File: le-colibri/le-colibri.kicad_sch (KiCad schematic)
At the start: 61 parts, among them SW1 CPG151101S11, SW10 CPG151101S11, SW11 CPG151101S11, SW12 CPG151101S11, SW13 CPG151101S11, SW14 CPG151101S11, SW15 CPG151101S11, SW16 CPG151101S11, SW17 CPG151101S11, SW18 CPG151101S11, SW19 CPG151101S11, SW2 CPG151101S11, SW20 CPG151101S11, SW21 CPG151101S11, SW22 CPG151101S11, SW23 CPG151101S11, SW24 CPG151101S11, SW25 CPG151101S11, SW26 CPG151101S11, SW27 CPG151101S11, SW28 CPG151101S11, SW29 CPG151101S11, SW3 CPG151101S11, SW30 CPG151101S11, SW4 CPG151101S11, SW5 CPG151101S11, SW6 CPG151101S11, SW7 CPG151101S11, SW8 CPG151101S11, SW9 CPG151101S11, U1 Seeeduino Xiao rp2040

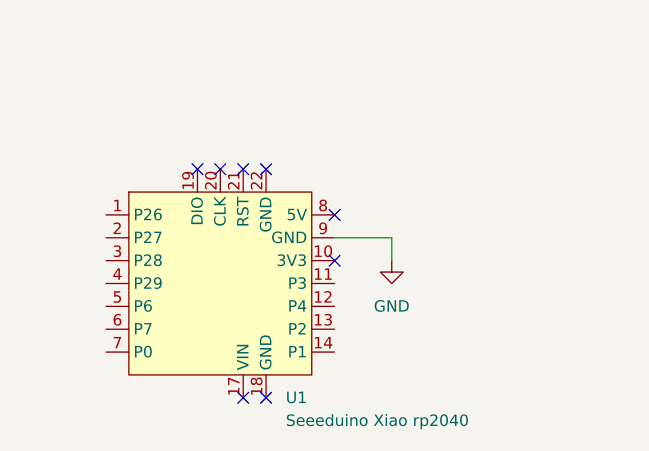
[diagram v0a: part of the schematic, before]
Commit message: "first" "release"
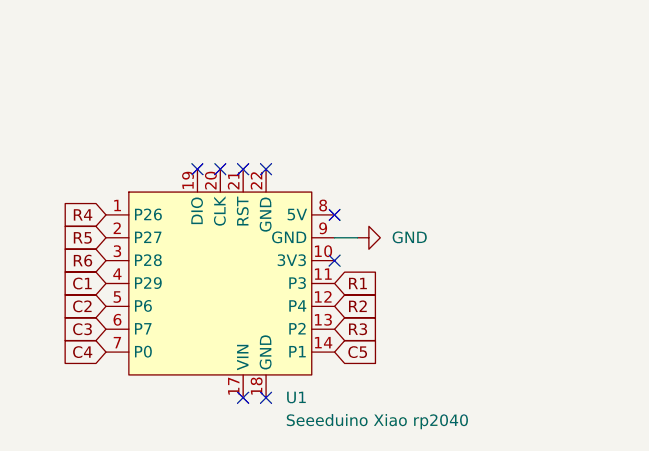
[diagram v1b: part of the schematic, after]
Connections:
- net C1: now also U1.4 (P29)
- net C2: now also U1.5 (P6)
- net C3: now also U1.6 (P7)
- net C4: now also U1.7 (P0)
- net C5: now also U1.14 (P1)
- net R1: now also U1.11 (P3)
- net R2: now also U1.12 (P4)
- net R3: now also U1.13 (P2)
- net R4: now also U1.1 (P26)
- net R5: now also U1.2 (P27)
- net R6: now also U1.3 (P28)
